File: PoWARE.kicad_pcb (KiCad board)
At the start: 4 copper layers, 30.4 x 51.3 mm, 49 parts, among them J1 Conn_02x03_Counter_Clockwise, J2 Conn_02x03_Counter_Clockwise, J3 Screw_Terminal_01x02, J4 Conn_02x01, J5 Conn_02x01, J6 Conn_02x01, J7 Conn_02x01, P1 USB_C_Plug_USB2.0, SW1 SW_SPDT, SW2 SW_SP4T, U1 SY8303AIC, U2 CH224K

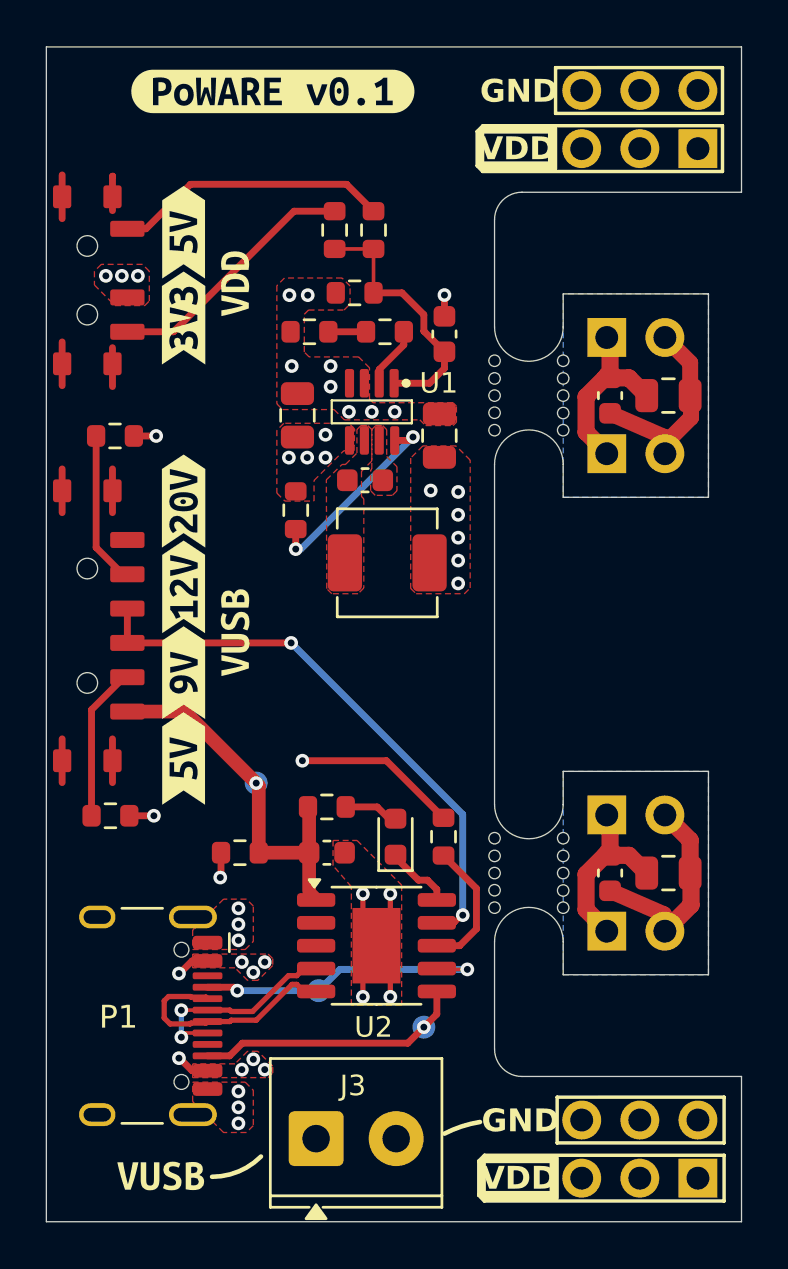
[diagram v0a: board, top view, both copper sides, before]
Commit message: Cleaned up repo
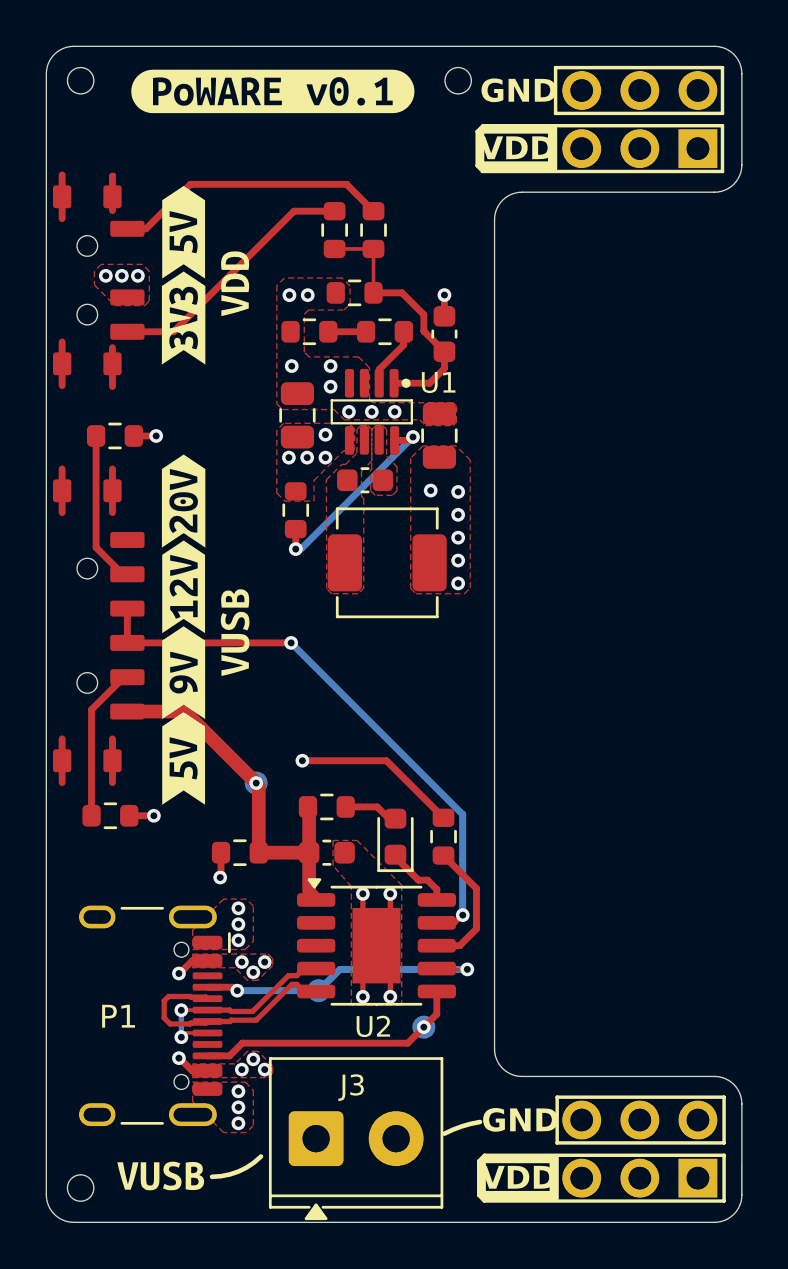
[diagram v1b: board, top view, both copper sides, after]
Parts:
- removed C11, C12: 10u, Capacitor_SMD:C_0805_2012Metric
- removed C7, C9: 100n, Capacitor_SMD:C_0603_1608Metric
- removed J4, J5, J6, J7: Conn_02x01, Connector_PinHeader_2.54mm:PinHeader_2x01_P2.54mm_Vertical
- removed mouse-bite-3mm-slot (x2): VAL**, Panelization:mouse-bite-3mm-slot
- added ?: , , F.Cu at (121.6, 77.1)
- added ?: , , F.Cu at (105.1, 77.1)
- added REF**: ToolingHole_1.152mm, MountingHole:ToolingHole_1.152mm, F.Cu at (105.1, 125.5)
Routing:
- net /B: track 9.51 -> 0.00 mm
- net /D: track 9.39 -> 0.00 mm
- net /A: track 8.00 -> 0.00 mm
- net /C: track 8.00 -> 0.00 mm
- removed copper zone on B.Cu, net /A
- removed copper zone on In1.Cu, net /A
- removed copper zone on In2.Cu, net /B
- removed copper zone on B.Cu, net /C
- removed copper zone on In1.Cu, net /C
- removed copper zone on In2.Cu, net /D
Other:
- board size 30.4 x 51.3 mm -> 30.4 x 51.4 mm
- board text removed: "BREAK OFF"
